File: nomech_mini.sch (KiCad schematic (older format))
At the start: 58 parts, among them CON1 USB_2B, CON2 AVR-ISP-6, P1 CONN_1, P2 CONN_1, P3 CONN_1, P4 CONN_1, P5 CONN_1, U1 ATMEGA32U4, X1 CRYSTAL_16MHz

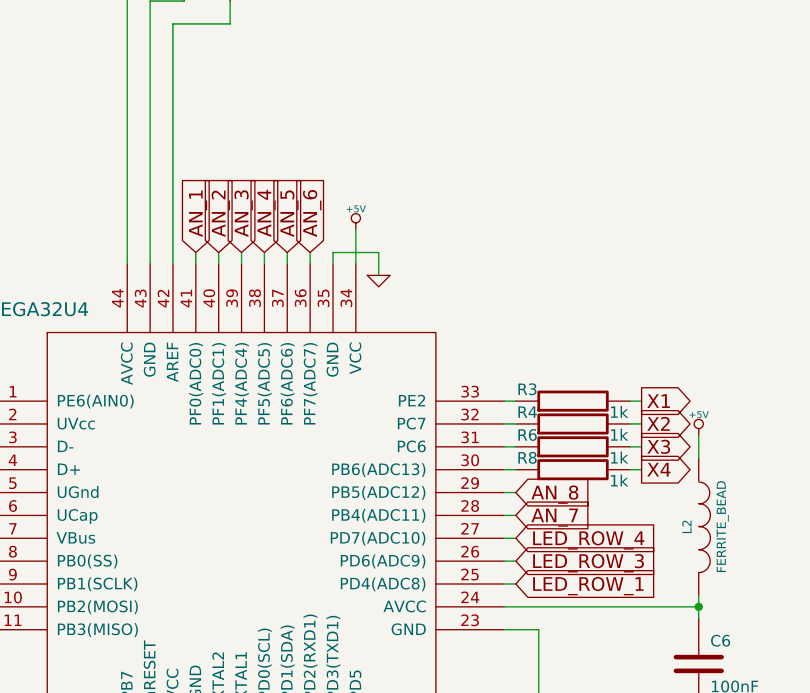
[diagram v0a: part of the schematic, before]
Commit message: routing...
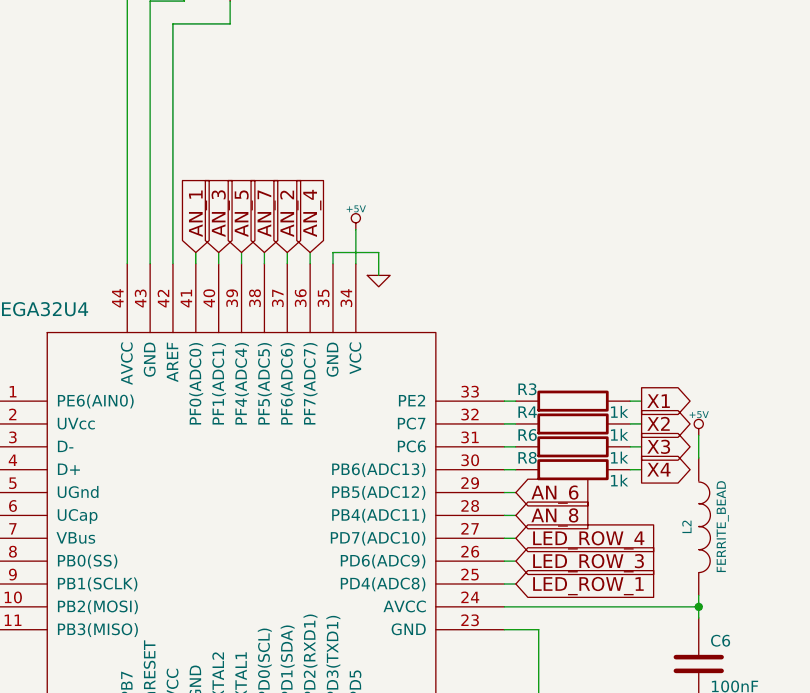
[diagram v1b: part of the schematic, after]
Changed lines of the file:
@@
-EESchema Schematic File Version 2  date Sat 04 May 2013 23:18:21 BST
+EESchema Schematic File Version 2  date Wed 08 May 2013 17:46:27 BST
 LIBS:power
 LIBS:device
@@
 Sheet 1 2
 Title ""
-Date "4 may 2013"
+Date "8 may 2013"
 Rev ""
 Comp ""
@@
 Text GLabel 4700 4050 1    60   Input ~ 0
 AN_1
+Text GLabel 5100 4050 1    60   Input ~ 0
+AN_2
 Text GLabel 4800 4050 1    60   Input ~ 0
-AN_2
-Text GLabel 4900 4050 1    60   Input ~ 0
 AN_3
-Text GLabel 5000 4050 1    60   Input ~ 0
+Text GLabel 5200 4050 1    60   Input ~ 0
 AN_4
 $Comp
@@
 Text GLabel 10750 5250 2    60   Input ~ 0
 Y2
-Text GLabel 5100 4050 1    60   Input ~ 0
+Text GLabel 4900 4050 1    60   Input ~ 0
 AN_5
-Text GLabel 5200 4050 1    60   Input ~ 0
+Text GLabel 6100 5100 2    60   Input ~ 0
 AN_6
-Text GLabel 6100 5200 2    60   Input ~ 0
+Text GLabel 5000 4050 1    60   Input ~ 0
 AN_7
 $Comp
@@
 Text GLabel 4100 6250 0    60   Output ~ 0
 SLOPE
-Text GLabel 6100 5100 2    60   Input ~ 0
+Text GLabel 6100 5200 2    60   Input ~ 0
 AN_8
 NoConn ~ 8050 5100
